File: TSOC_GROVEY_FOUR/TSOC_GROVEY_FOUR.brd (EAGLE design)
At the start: 44.5 x 30.5 mm, 39 parts, among them J2 JTAG-ISSPMIN, J3 4P-2.0-90D, J4 4P-2.0-90D, J5 4P-2.0-90D, J6 4P-2.0-90D, U1 CY8C4XXX-28

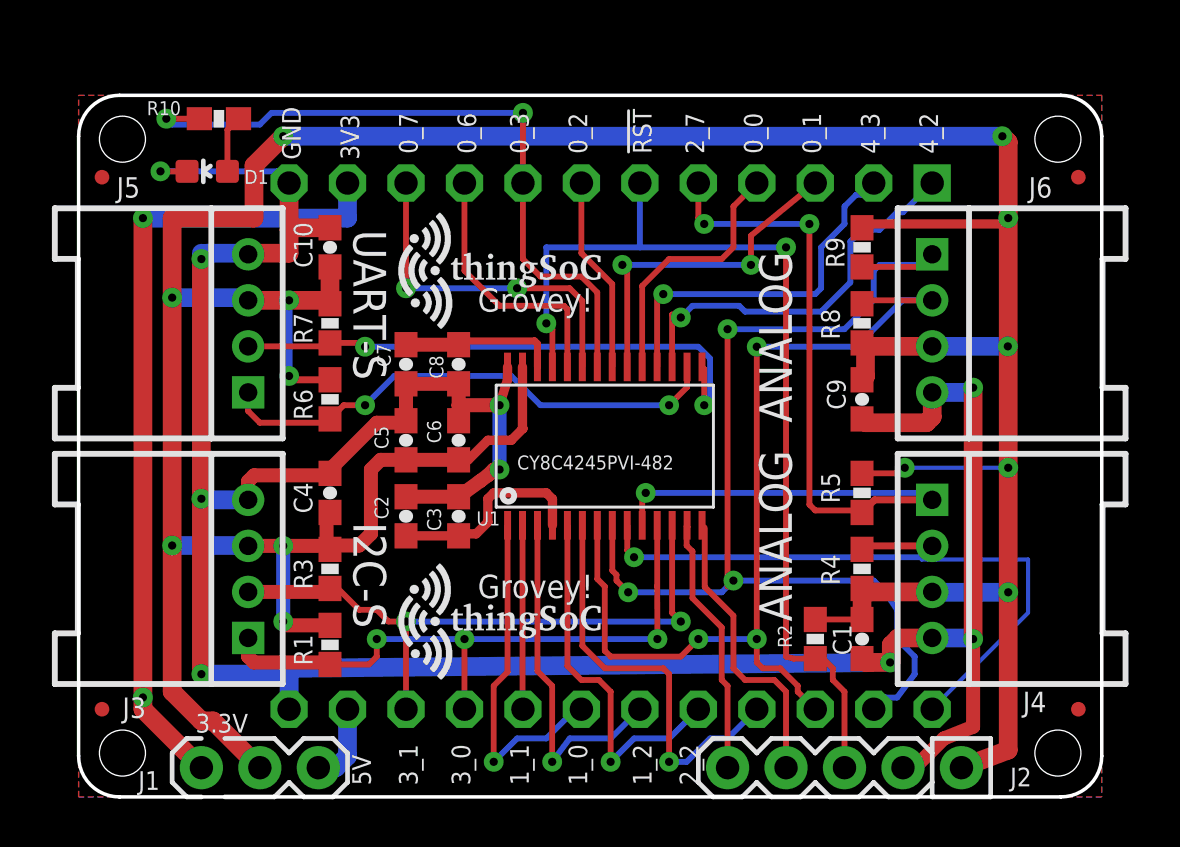
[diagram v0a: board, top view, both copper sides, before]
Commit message: update Rev 3.0
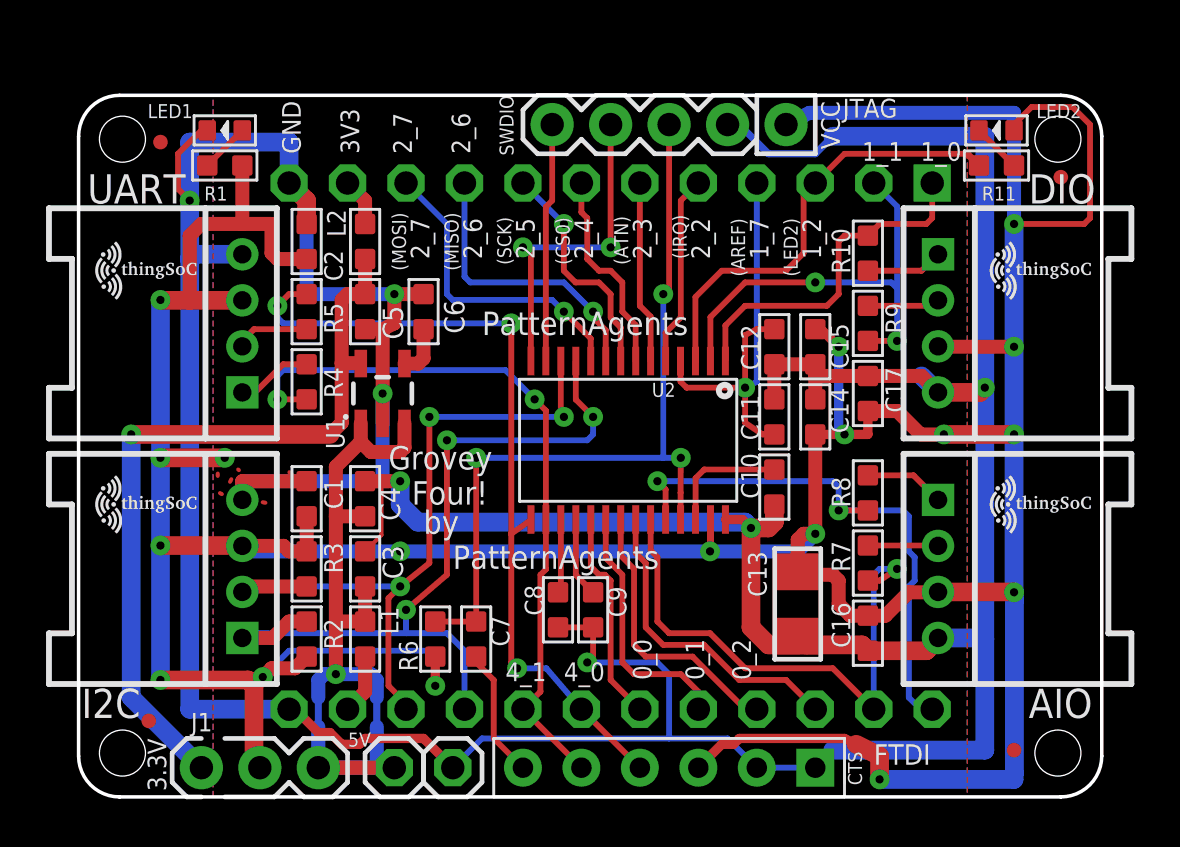
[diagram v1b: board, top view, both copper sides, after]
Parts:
- removed D1: (no value), TSOC-ESP8266-BASE:LED-0603
- removed J2: JTAG-ISSPMIN, PatternAgents-Cypress:PSOC_JTAG_MINSILK
- removed J3, J4, J5, J6: 4P-2.0-90D, Seeed-Connector -2016:HW4-2.0-90D
- removed U$101: TSOC-LOGO-LRG, thingSoC:TSOC-LOGO-LRG
- added $$U$2, $$U$3, U$103: TSOC-LOGO-SMALL, thingSoC:TSOC-LOGO-SML
- added 5V0, GND: (no value), PatternAgents-ProtoPads:1X01
- added AIO, DIO, I2C, UART: 4P-2.0-90D, Seeed-Connector -2016:HW4-2.0-90D
- added C11, C15, C16, C17: 100nf, Seeed-Capacitor-2016:C0603
- added C12, C14: 1uF, Seeed-Capacitor-2016:C0603
- added C13: 22uF, TSOC_USBUART2:EIA-1206
- added FTDI: 6p-2.54, Seeed-Connector -2016:H6-2.54
- added JTAG: JTAG-ISSPMIN, PatternAgents-Cypress:PSOC_JTAG_MINSILK
- added L1, L2: 120OHM-500MA, Seeed-Inductor-2016:L0603
- added LED1: GREEN-0603, Seeed-LED-2016:LED-0603
- added LED2: RED-0603, Seeed-LED-2016:LED-0603
- added R11: 1K 1/10W, Seeed-Resistor-2016:R0603
- added TSOC: TSOC-24-BB, thingSoC:TSOC-BB-S24
- added U2: CY8C4XXX-28, PatternAgents-Cypress:SSOP28
- C1, C4: value 1uF -> 100nf; device SparkFun-Passives:0603-CAP -> Seeed-Capacitor-2016:C0603
- C10: device SparkFun-Passives:0603-CAP -> Seeed-Capacitor-2016:C0603
- C2, C7: value 1uF -> 100nf; device PatternAgents-Misc:0603-CAP -> Seeed-Capacitor-2016:C0603
- C3: value 0.1uF -> 10uf; device PatternAgents-Misc:0603-CAP -> Seeed-Capacitor-2016:C0603
- C5: value 1uF -> 10uf; device PatternAgents-Misc:0603-CAP -> Seeed-Capacitor-2016:C0603
- C6: value 0.1uF -> 470Pf; device PatternAgents-Misc:0603-CAP -> Seeed-Capacitor-2016:C0603
- C8: value 0.1uF -> 2.2nf; device PatternAgents-Misc:0603-CAP -> Seeed-Capacitor-2016:C0603
- C9: value 1uF -> 10nf; device SparkFun-Passives:0603-CAP -> Seeed-Capacitor-2016:C0603
- J1: value (none) -> NO
- R1: value 2k2 -> 1K 1/10W; device SparkFun-Passives:0603-RES -> Seeed-Resistor-2016:R0603
- R10: device PatternAgents-Misc:0603-RES -> Seeed-Resistor-2016:R0603
- R2: value 10K -> 2.2K; device PatternAgents-Misc:0603-RES -> Seeed-Resistor-2016:R0603
- R3: value 2k2 -> 2.2K; device SparkFun-Passives:0603-RES -> Seeed-Resistor-2016:R0603
- R4, R5, R8, R9: value 2k2 -> 1K; device SparkFun-Passives:0603-RES -> Seeed-Resistor-2016:R0603
- R6: value DNP -> 10K 1/10W; device SparkFun-Passives:0603-RES -> Seeed-Resistor-2016:R0603
- R7: value DNP -> 1K; device SparkFun-Passives:0603-RES -> Seeed-Resistor-2016:R0603
- U$1: value TSOC-LOGO-MED -> TSOC-LOGO-SMALL; device thingSoC:TSOC-LOGO-MED -> thingSoC:TSOC-LOGO-SML
- U$102: value TSOC-LOGO-SMALL -> TSOC-LOGO-LRG; device thingSoC:TSOC-LOGO-SML -> thingSoC:TSOC-LOGO-LRG
- U$3: value TSOC-24-BB -> TSOC-LOGO-SMALL; device thingSoC:TSOC-BB-S24 -> thingSoC:TSOC-LOGO-SML
- U$4: value TSOC-LOGO-MED -> TSOC-LOGO; device thingSoC:TSOC-LOGO-MED -> thingSoC:TSOC-LOGO-BLANK
- U1: value CY8C4XXX-28 -> MIC5219 3.3V; device PatternAgents-Cypress:SSOP28 -> TSOC-ESP8266-BASE:SOT23-5
- moved FID2 46.9 mm to (3.56, 28.4)
- moved FID3 46.8 mm to (40.6, 2.03)
- moved U$100 39.6 mm to (4.32, 15.2)
- moved R10 28.8 mm to (34.3, 23.6), turned to 0 degrees
- moved U$4 27.6 mm to (0.00, 0.00)
- moved U$102 26.6 mm to (31.2, 16.8)
- moved R7 25.6 mm to (34.3, 10.2), turned to 180 degrees
- moved R4 25.5 mm to (9.91, 18.0), turned to 180 degrees
- moved R5 25.4 mm to (9.91, 21.1), turned to 0 degrees
- moved U$3 25.3 mm to (1.52, 22.9), turned to 0 degrees
- moved C1 24.9 mm to (9.91, 13.0), turned to 180 degrees
- moved R2 22.1 mm to (9.91, 6.86), turned to 0 degrees
- moved C10 21.9 mm to (30.2, 13.5), turned to 180 degrees
- moved R1 21.3 mm to (6.35, 27.4)
- moved U$1 14.9 mm to (1.52, 12.7)
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- renumbered U$2 to $$U$1
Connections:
- new net !URST: C7.1, FTDI.6
- new net BYPASS1: C6.1, U1.4
- new net LEDR: LED2.-, R11.1
- new net P0_6E: AIO.2, R7.2
- new net P0_7E: AIO.1, R8.2
- new net P1_0E: DIO.1, R10.2
- new net P1_1E: DIO.2, R9.2
- new net P4_0E: R5.2, UART.2
- new net P4_1E: R4.2, UART.1
- new net TSOC_3V3: L2.2, TSOC.11B
- new net TSOC_5V0: L1.2, TSOC.11C
- net !XRES: now also C7.2, JTAG.3, R6.1, U2.25; no longer J2.3, R2.1, U$3.6B, U1.25
- net 3V3: now also C5.2, L2.1, U1.5; no longer U$3.11B
- net 5V0: now also 5V0.1, C3.2, C4.1, L1.1, U1.1, U1.3; no longer U$3.11C
- net GND: now also AIO.4, C10.1, C11.1, C12.1, C13.2, C14.1, C15.1, C16.2, C17.2, C3.1, C5.1, C8.1, C9.1, DIO.4, FTDI.1, FTDI.2, GND.1, I2C.4, JTAG.2, LED1.-, TSOC.12B, TSOC.12C, U1.2, U2.28, UART.4; no longer C10.2, C3.2, C5.2, C7.2, C8.2, C9.2, D1.C, J2.2, J3.4, J4.4, J5.4, J6.4, U$3.12B, U$3.12C, U1.28
- net N$17: now also LED1.+, R1.1; no longer D1.A, R10.1
- net P0_0: now also TSOC.6C, U2.19; no longer U$3.4B, U1.19
- net P0_1: now also TSOC.5C, U2.20; no longer U$3.3B, U1.20
- net P0_2: now also TSOC.4C, U2.21; no longer U$3.7B, U1.21
- net P0_3: now also TSOC.3C, U2.22; no longer R10.2, U$3.8B, U1.22
- net P0_6: now also R7.1, TSOC.2C, U2.23; no longer U$3.9B, U1.24
- net P0_7: now also R8.1, TSOC.1C, U2.24; no longer U$3.10B, U1.23
- net P1_0: now also R10.1, TSOC.1B, U2.1; no longer U$3.7C, U1.1
- net P1_1: now also R9.1, TSOC.2B, U2.2; no longer U$3.8C, U1.2
- net P1_2: now also R11.2, TSOC.3B, U2.3; no longer U$3.6C, U1.3
- net P1_7: now also C11.2, C12.2, TSOC.4B, U2.4; no longer C2.1, C3.1, U1.4
- net P2_2: now also TSOC.5B, U2.5; no longer U$3.5C, U1.5
- net P2_3: now also TSOC.6B, U2.6; no longer U$3.4C, U1.6
- net P2_4: now also TSOC.7B, U2.7; no longer J6.2, R8.1, U$3.3C, U1.7
- net P2_5: now also TSOC.8B, U2.8; no longer J6.1, R9.1, U$3.2C, U1.8
- net P2_6: now also TSOC.9B, U2.9; no longer J4.2, R4.1, U$3.1C, U1.9
- net P2_7: now also TSOC.10B, U2.10; no longer J4.1, R5.1, U$3.5B, U1.10
- net P3_0: now also I2C.1, R2.1, TSOC.9C, U2.11; no longer J3.1, R1.1, U$3.9C, U1.11
- net P3_1: now also I2C.2, TSOC.10C, U2.12; no longer J3.2, U$3.10C, U1.12
- net P3_2: now also JTAG.5, U2.13; no longer J2.5, U1.13
- net P3_3: now also JTAG.4, U2.14; no longer J2.4, U1.14
- net P4_0: now also FTDI.4, R5.1, TSOC.7C, U2.15; no longer J5.2, R7.1, U1.15
- net P4_1: now also FTDI.5, R4.1, TSOC.8C, U2.16; no longer J5.1, R6.1, U1.16
- net P4_2: now also C8.2, U2.17; no longer U$3.1B, U1.17
- net P4_3: now also C9.2, U2.18; no longer U$3.2B, U1.18
- net VCC: now also AIO.3, C13.1, C14.2, C15.2, C16.1, C17.1, C2.1, DIO.3, FTDI.3, I2C.3, JTAG.1, LED2.+, U2.27, UART.3; no longer C10.1, C4.1, C5.1, C6.1, C9.1, J2.1, J3.3, J4.3, J5.3, J6.3, R4.2, R5.2, R7.2, R8.2, R9.2, U1.27
- net VCCD: now also C10.2, U2.26; no longer C7.1, C8.1, U1.26
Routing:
- net GND: track 125.6 -> 213.4 mm, vias 9 -> 7
- net P2_5: track 47.2 -> 10.1 mm, vias 3 -> 1
- net 5V0: track 3.51 -> 38.9 mm, vias 0 -> 1
- net P2_4: track 41.4 -> 9.01 mm, vias 3 -> 0
- net VCC: track 167.7 -> 194.8 mm, vias 13 -> 18
- net P2_7: track 38.4 -> 13.6 mm, vias 3 -> 1
- net P2_6: track 30.7 -> 12.7 mm
- net P0_3: track 30.7 -> 13.7 mm, vias 2 -> 0
- net P4_2: track 17.3 -> 3.21 mm, vias 1 -> 0
- net P4_3: track 16.0 -> 3.47 mm, vias 1 -> 0
- net P0_6: track 11.5 -> 23.9 mm, vias 0 -> 1
- net P4_0: track 24.2 -> 35.6 mm, vias 2 -> 3
- net P1_1: track 8.00 -> 19.3 mm, vias 0 -> 2
- net P1_7: track 8.98 -> 19.6 mm, vias 0 -> 1
- net P2_3: track 18.1 -> 7.93 mm, vias 1 -> 0
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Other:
- board text added: "(AREF)"
- board text added: "(ATN)"
- board text added: "(CS0)"
- board text added: "(IRQ)"
- board text added: "(LED2)"
- board text added: "(MISO)"
- board text added: "(MOSI)"
- board text added: "(SCK)"
- board text added: "1_7"
- board text added: "4_0"
- board text added: "4_1"
- board text added: "AIO"
- board text added: "DIO"
- board text added: "FTDI"
- board text added: "Four!"
- board text added: "Grovey"
- board text added: "I2C"
- board text added: "J1"
- board text added: "JTAG"
- board text added: "P0_6"
- board text added: "P0_7"
- board text added: "P1_0"
- board text added: "P1_1"
- board text added: "Rev. 3.0"
- board text added: "SWC"
- board text added: "SWD"
- board text added: "SWDIO"
- board text added: "TSOC_GROVEY_FOUR!"
- board text added: "UART"
- board text added: "by"
- board text removed: "!CS"
- board text removed: "!DCD"
- board text removed: "!DSR"
- board text removed: "!IRQ"
- board text removed: "!RI"
- board text removed: "!RTS"
- board text removed: "0_7"
- board text removed: "4_2"
- board text removed: "4_3"
- board text removed: "ANALOG"
- board text removed: "CY8C4245PVI-482"
- board text removed: "Grovey!"
- board text removed: "I2C-S"
- board text removed: "IO1"
- board text removed: "IO2"
- board text removed: "J2"
- board text removed: "MISO"
- board text removed: "MOSI"
- board text removed: "P2_4"
- board text removed: "P2_5"
- board text removed: "P2_6"
- board text removed: "P2_7"
- board text removed: "Rev. 2.0"
- board text removed: "SCK"
- board text removed: "SCL"
- board text removed: "SDA"
- board text removed: "SS1"
- board text removed: "SS2"
- board text removed: "UART-S"
